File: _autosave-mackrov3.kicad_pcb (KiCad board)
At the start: 2 copper layers, 97.4 x 54.1 mm, 31 parts, among them U1 ProMicro

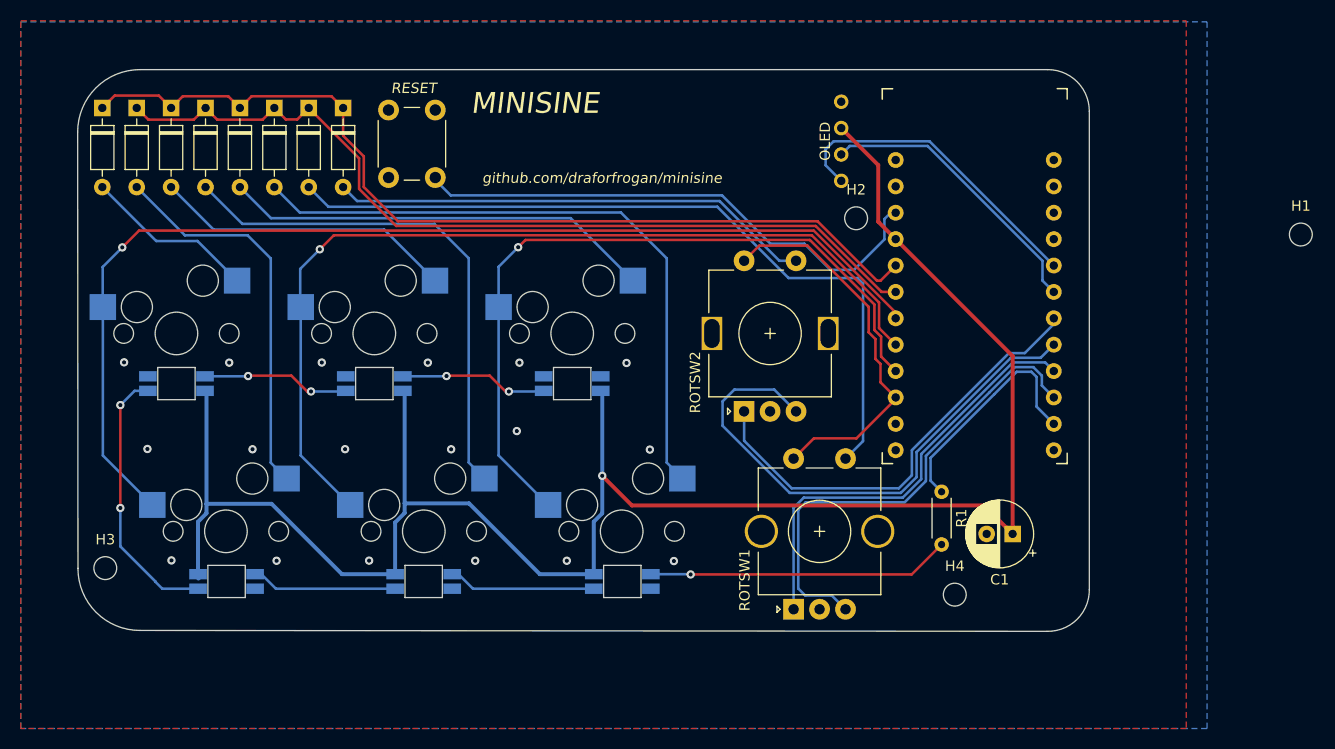
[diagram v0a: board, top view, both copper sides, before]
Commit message: Add updates
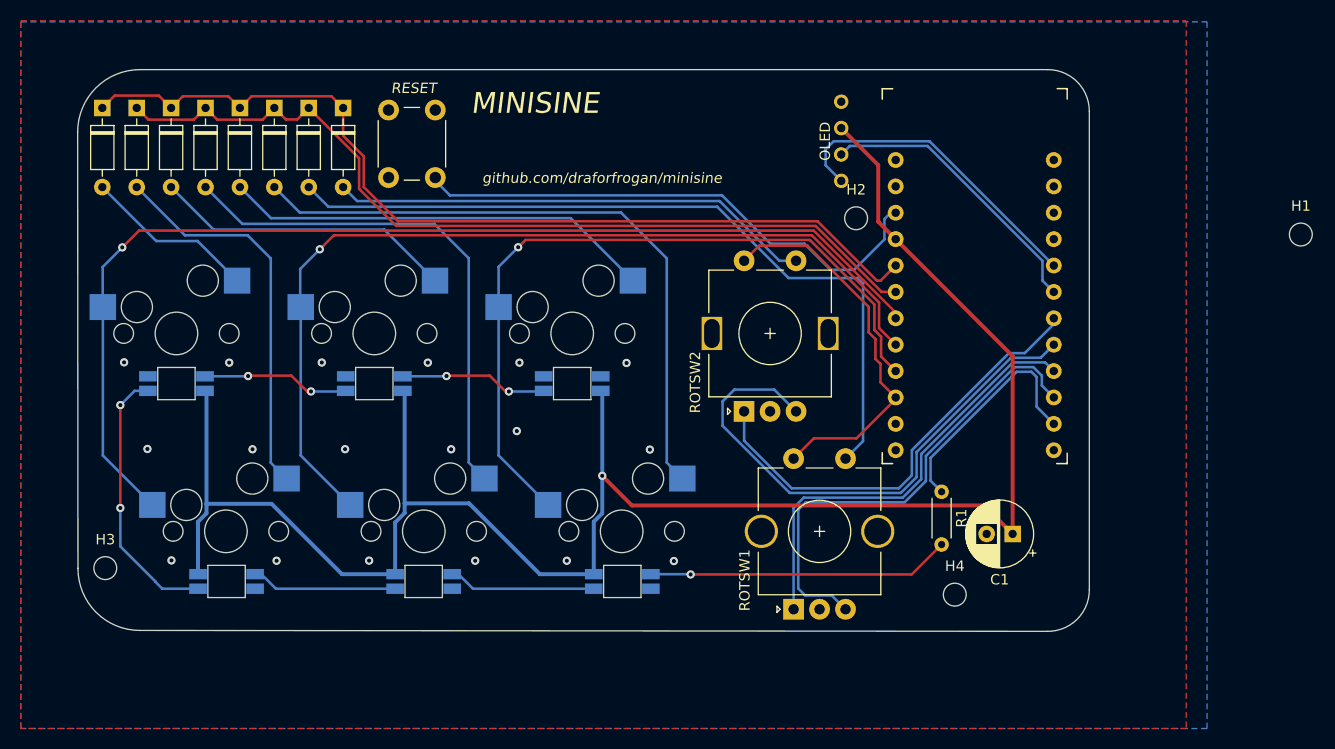
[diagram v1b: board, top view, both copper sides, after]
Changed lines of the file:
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@@
       (drillshape 0)
       (scaleselection 1)
-      (outputdirectory "../../../Desktop/mackro2/")
+      (outputdirectory "C:/Users/ziggy/Desktop/mckc3/")
     )
   )
@@
   (gr_line (start 265.679885 64.220303) (end 265.683999 110.236) (layer "Edge.Cuts") (width 0.1))
   (gr_line (start 261.61516 114.275808) (end 174.3 114.189999) (layer "Edge.Cuts") (width 0.1))
-  (gr_arc (start 174.3 114.189999) (mid 170.065246 112.444005) (end 168.320004 108.20894) (layer "Edge.Cuts") (width 0.1))
+  (gr_arc (start 174.3 114.189999) (mid 170.065245 112.444005) (end 168.320004 108.20894) (layer "Edge.Cuts") (width 0.1))
   (gr_arc (start 261.69 60.2) (mid 264.52205 61.379378) (end 265.679885 64.220303) (layer "Edge.Cuts") (width 0.1))
   (gr_rect (start 265.67 110.27) (end 261.67 114.27) (layer "User.4") (width 0.15) (fill none))
@@
   (segment (start 250.4 99.778) (end 251.46 100.838) (width 0.25) (layer "B.Cu") (net 18))
   (segment (start 260.604 89.789718) (end 260.104036 89.289754) (width 0.25) (layer "B.Cu") (net 18))
-  (segment (start 258.690247 89.289754) (end 256.53048 91.44952) (width 0.25) (layer "B.Cu") (net 18))
   (segment (start 250.4 97.58) (end 250.4 99.778) (width 0.25) (layer "B.Cu") (net 18))
-  (segment (start 256.53048 91.44952) (end 250.4 97.58) (width 0.25) (layer "B.Cu") (net 18))
+  (segment (start 250.4 97.58) (end 258.690247 89.289754) (width 0.25) (layer "B.Cu") (net 18))
   (segment (start 262.2614 94.300714) (end 260.604 92.643314) (width 0.25) (layer "B.Cu") (net 18))
   (segment (start 260.104036 89.289754) (end 258.690247 89.289754) (width 0.25) (layer "B.Cu") (net 18))
@@
   (segment (start 244.44096 83.037412) (end 244.440961 85.493131) (width 0.25) (layer "F.Cu") (net 22))
   (segment (start 239.1645 95.7) (end 237.2125 97.652) (width 0.25) (layer "F.Cu") (net 22))
+  (segment (start 202.72 70.59) (end 202.72 70.894) (width 0.25) (layer "B.Cu") (net 24))
+  (segment (start 245.954889 76.545111) (end 245.954889 74.585111) (width 0.25) (layer "B.Cu") (net 24))
+  (segment (start 204.12984 72.30384) (end 230.322117 72.303841) (width 0.25) (layer "B.Cu") (net 24))
+  (segment (start 243.023009 79.476991) (end 245.954889 76.545111) (width 0.25) (layer "B.Cu") (net 24))
   (segment (start 234.980276 76.962) (end 238.252 76.962) (width 0.25) (layer "B.Cu") (net 24))
-  (segment (start 204.20384 72.30384) (end 230.322117 72.303841) (width 0.25) (layer "B.Cu") (net 24))
   (segment (start 246.559286 73.980714) (end 247.0414 73.980714) (width 0.25) (layer "B.Cu") (net 24))
   (segment (start 230.322117 72.303841) (end 234.980276 76.962) (width 0.25) (layer "B.Cu") (net 24))
-  (segment (start 202.75 70.85) (end 204.20384 72.30384) (width 0.25) (layer "B.Cu") (net 24))
-  (segment (start 245.954889 76.545111) (end 245.954889 74.585111) (width 0.25) (layer "B.Cu") (net 24))
-  (segment (start 243.023009 79.476991) (end 245.954889 76.545111) (width 0.25) (layer "B.Cu") (net 24))
   (segment (start 245.954889 74.585111) (end 246.559286 73.980714) (width 0.25) (layer "B.Cu") (net 24))
   (segment (start 238.252 76.962) (end 240.766991 79.476991) (width 0.25) (layer "B.Cu") (net 24))
   (segment (start 240.766991 79.476991) (end 243.023009 79.476991) (width 0.25) (layer "B.Cu") (net 24))
+  (segment (start 202.72 70.894) (end 204.12984 72.30384) (width 0.25) (layer "B.Cu") (net 24))
   (segment (start 172.585 77.315) (end 174.20096 75.69904) (width 0.25) (layer "F.Cu") (net 26))
   (segment (start 239.151161 75.69904) (end 247.0414 83.589279) (width 0.25) (layer "F.Cu") (net 26))
@@
   (segment (start 260.290234 88.840234) (end 258.504049 88.840234) (width 0.25) (layer "B.Cu") (net 30))
   (segment (start 237.66202 102.571698) (end 237.66202 110.15402) (width 0.25) (layer "B.Cu") (net 30))
-  (segment (start 258.504049 88.840234) (end 256.08096 91.263322) (width 0.25) (layer "B.Cu") (net 30))
   (segment (start 262.2614 91.760714) (end 261.112 90.611314) (width 0.25) (layer "B.Cu") (net 30))
   (segment (start 249.95048 99.80752) (end 247.904 101.854) (width 0.25) (layer "B.Cu") (net 30))
@@
   (segment (start 247.904 101.854) (end 238.379718 101.854) (width 0.25) (layer "B.Cu") (net 30))
   (segment (start 238.379718 101.854) (end 237.66202 102.571698) (width 0.25) (layer "B.Cu") (net 30))
-  (segment (start 256.08096 91.263322) (end 249.95048 97.393803) (width 0.25) (layer "B.Cu") (net 30))
+  (segment (start 249.95048 97.393803) (end 258.504049 88.840234) (width 0.25) (layer "B.Cu") (net 30))
   (segment (start 247.717802 101.40448) (end 249.50096 99.621322) (width 0.25) (layer "B.Cu") (net 31))
   (segment (start 258.317851 88.390714) (end 261.4314 88.390714) (width 0.25) (layer "B.Cu") (net 31))
@@
   (segment (start 212.784288 108.774) (end 205.970288 101.96) (width 0.381) (layer "B.Cu") (net 37))
   (segment (start 186.957767 101.997479) (end 180.692521 101.997479) (width 0.381) (layer "B.Cu") (net 37))
-  (segment (start 179.912 109.2) (end 180.138 108.974) (width 0.381) (layer "B.Cu") (net 37))
   (segment (start 180.692521 101.997479) (end 180.692521 91.266521) (width 0.381) (layer "B.Cu") (net 37))
   (segment (start 218.792521 99.302521) (end 218.792521 91.266521) (width 0.381) (layer "B.Cu") (net 37))
